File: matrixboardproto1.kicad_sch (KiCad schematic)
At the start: 11 parts, among them Q1 BC107, SW1 SW_Push

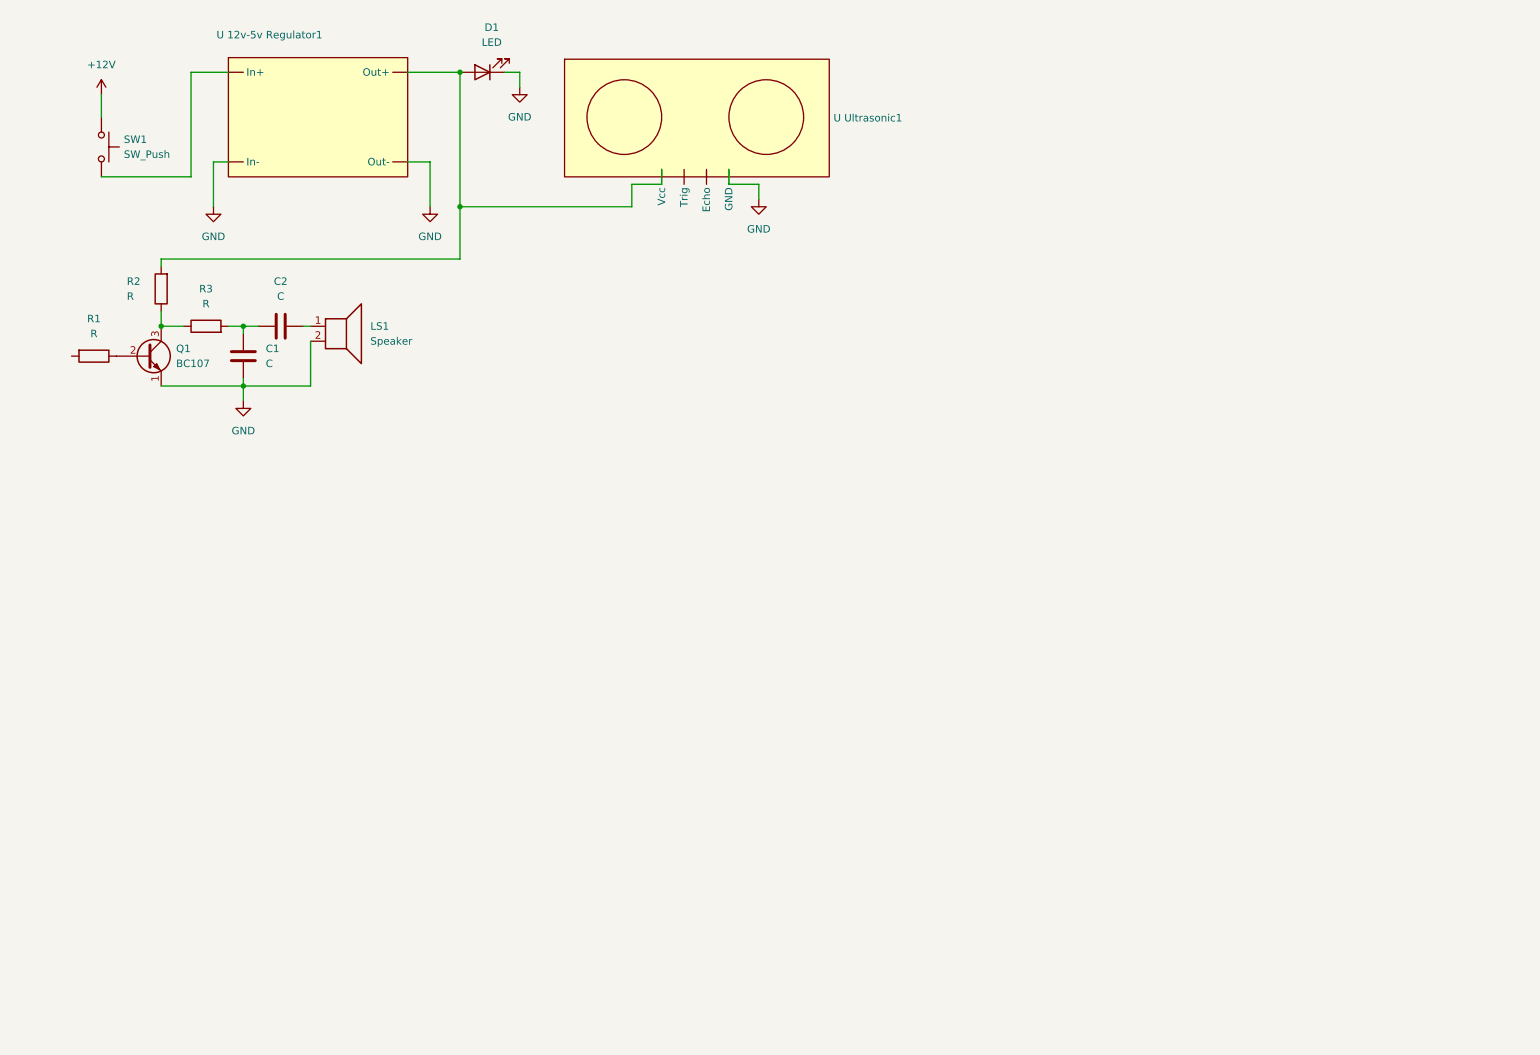
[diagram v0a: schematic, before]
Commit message: Add files via upload
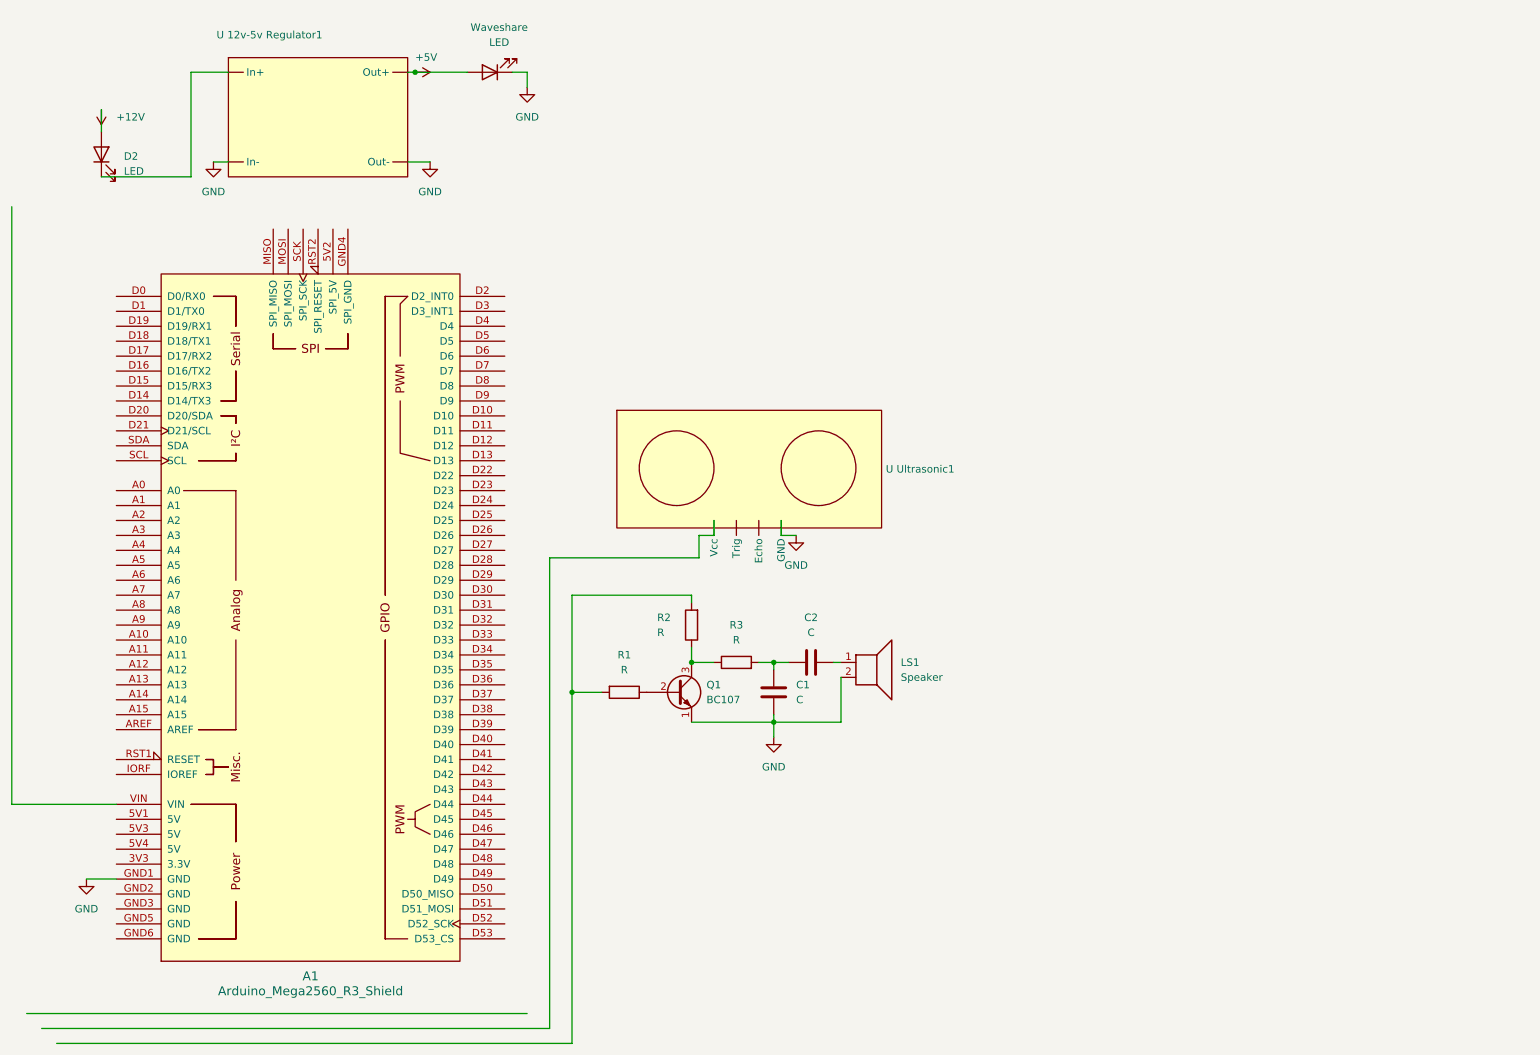
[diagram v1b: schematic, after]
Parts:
- removed SW1: SW_Push, symbol Switch:SW_Push
- added A1: Arduino_Mega2560_R3_Shield, PCM_arduino-library:Arduino_Mega2560_R3_Shield, symbol arduino-library:Arduino_Mega2560_R3_Shield
- added D2: LED, symbol Device:LED
- renumbered D1 to Waveshare
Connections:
- net +12V: now also D2.2 (A)
- net GND: now also A1.GND1 (GND)
- net at R1.2: now also R2.2
- new net: D2.1 (K), U 12v-5v Regulator1. (Out-)
- new net +5V: U 12v-5v Regulator1. (Out-), Waveshare.2 (A)
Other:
- moved on the sheet: C1, C2, LS1, Q1, R1, R2, R3, U Ultrasonic1, Waveshare

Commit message: Add files via upload
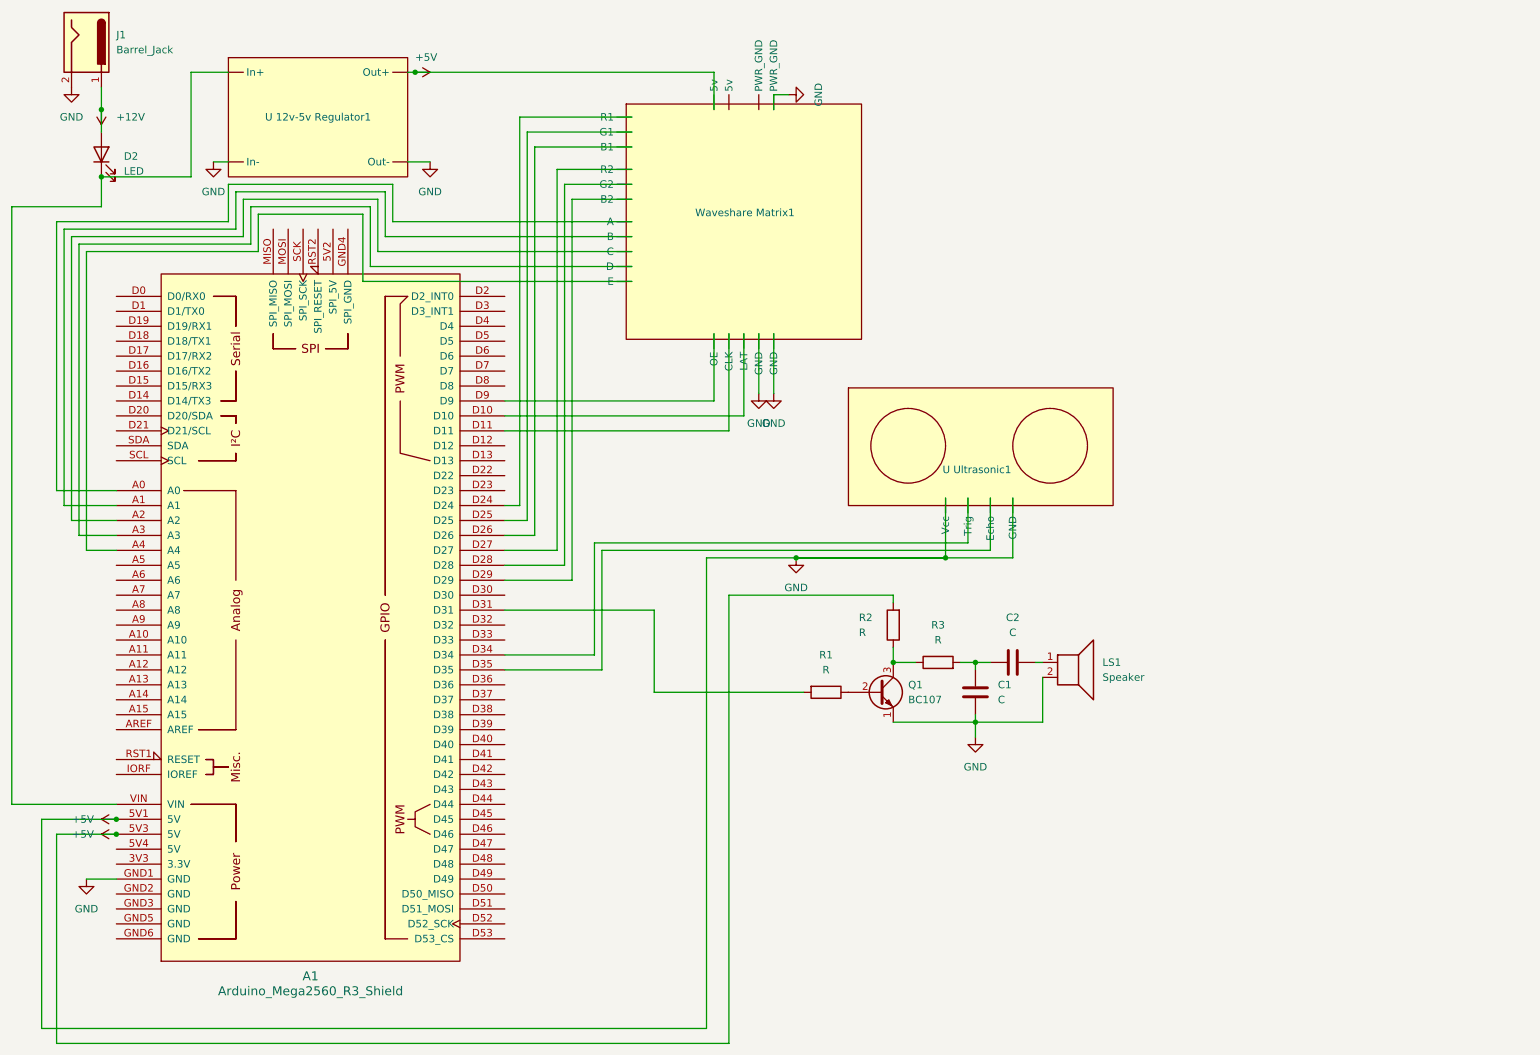
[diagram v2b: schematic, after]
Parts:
- removed Waveshare: LED, symbol Device:LED
- added J1: Barrel_Jack, symbol Connector:Barrel_Jack
- added Waveshare Matrix1: Waveshare Matrix, Waveshare Matrix, symbol Matrix_Board_Lib:Waveshare_LED_Matrix
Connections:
- net GND is gone; now on net +5V: A1.GND1 (GND), C1.1, LS1.2, Q1.1 (E), U 12v-5v Regulator1. (Out-), U Ultrasonic1. (Vcc)
- net +12V: now also J1.1
- net +5V: now also A1.5V1 (5V), A1.5V3 (5V), R2.2, J1.2, Waveshare Matrix1. (R2)
- net at D2.1 (K), U 12v-5v Regulator1. (Out-): now also A1.VIN
- net at R1.2: now also A1.D31; no longer R2.2
- net at A1.A0: now also Waveshare Matrix1. (R2)
- net at A1.A1: now also Waveshare Matrix1. (R2)
- net at A1.A2: now also Waveshare Matrix1. (R2)
- net at A1.A3: now also Waveshare Matrix1. (R2)
- net at A1.A4: now also Waveshare Matrix1. (R2)
- net at A1.D10: now also Waveshare Matrix1. (R2)
- net at A1.D11: now also Waveshare Matrix1. (R2)
- net at A1.D24: now also Waveshare Matrix1. (R2)
- net at A1.D25: now also Waveshare Matrix1. (R2)
- net at A1.D26: now also Waveshare Matrix1. (R2)
- net at A1.D27: now also Waveshare Matrix1. (R2)
- net at A1.D28: now also Waveshare Matrix1. (R2)
- net at A1.D29: now also Waveshare Matrix1. (R2)
- net at A1.D34: now also U Ultrasonic1. (Vcc)
- net at A1.D35: now also U Ultrasonic1. (Vcc)
- net at A1.D9: now also Waveshare Matrix1. (R2)
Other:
- moved on the sheet: C1, C2, LS1, Q1, R1, R2, R3, U Ultrasonic1

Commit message: Add files via upload
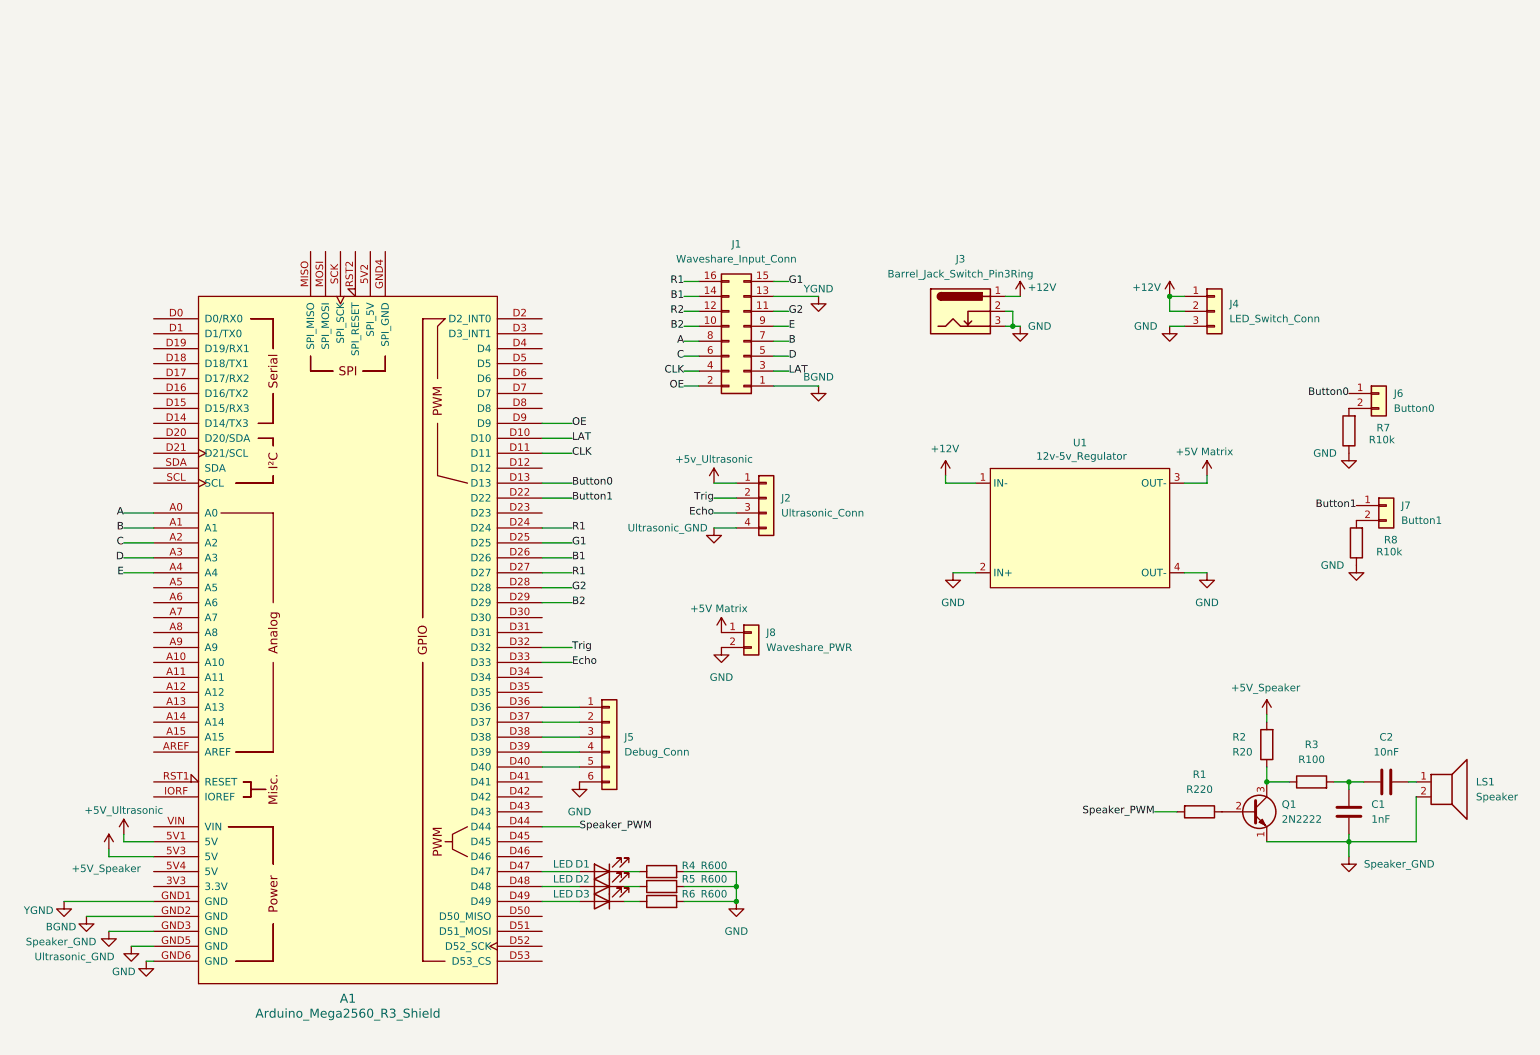
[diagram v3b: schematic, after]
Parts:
- removed J1: Barrel_Jack, symbol Connector:Barrel_Jack
- removed U 12v-5v Regulator1: ~, symbol Matrix_Board_Lib:DFR0831
- removed U Ultrasonic1: ~, symbol Matrix_Board_Lib:HCSR04_
- removed Waveshare Matrix1: Waveshare Matrix, Waveshare Matrix, symbol Matrix_Board_Lib:Waveshare_LED_Matrix
- added D1, D3: LED, LED_THT:LED_D5.0mm_Horizontal_O6.35mm_Z15.0mm, symbol Device:LED
- added J1: Waveshare_Input_Conn, Connector_IDC:IDC-Header_2x08_P2.54mm_Vertical, symbol Connector_Generic:Conn_02x08_Odd_Even
- added J2: Ultrasonic_Conn, Connector_PinHeader_1.00mm:PinHeader_1x04_P1.00mm_Vertical, symbol Connector_Generic:Conn_01x04
- added J3: Barrel_Jack_Switch_Pin3Ring, Connector_BarrelJack:BarrelJack_GCT_DCJ200-10-A_Horizontal, symbol Connector:Barrel_Jack_Switch_Pin3Ring
- added J4: LED_Switch_Conn, Connector:FanPinHeader_1x03_P2.54mm_Vertical, symbol Connector_Generic:Conn_01x03
- added J5: Debug_Conn, symbol Connector_Generic:Conn_01x06
- added J6: Button0, Connector_PinHeader_1.00mm:PinHeader_1x02_P1.00mm_Vertical, symbol Connector_Generic:Conn_01x02
- added J7: Button1, Connector_PinHeader_1.00mm:PinHeader_1x02_P1.00mm_Vertical, symbol Connector_Generic:Conn_01x02
- added J8: Waveshare_PWR, Connector_PinHeader_1.00mm:PinHeader_1x02_P1.00mm_Vertical, symbol Connector_Generic:Conn_01x02
- added R4, R5, R6: R600, Resistor_SMD:R_0805_2012Metric_Pad1.20x1.40mm_HandSolder, symbol Device:R
- added R7, R8: R10k, Resistor_SMD:R_0805_2012Metric_Pad1.20x1.40mm_HandSolder, symbol Device:R
- added U1: ~, matrixboard:DFR_Regulator, symbol Matrix_Board_Lib:DFR0831
- C1: value C -> 1nF; footprint (none) -> Capacitor_SMD:C_0805_2012Metric_Pad1.18x1.45mm_HandSolder
- C2: value C -> 10nF; footprint (none) -> Capacitor_SMD:C_0805_2012Metric_Pad1.18x1.45mm_HandSolder
- D2: footprint (none) -> LED_THT:LED_D5.0mm_Horizontal_O6.35mm_Z15.0mm
- LS1: footprint (none) -> Buzzer_Beeper:Speaker_CUI_CMR-1206S-67
- Q1: value BC107 -> 2N2222
- R1: value R -> R220; footprint (none) -> Resistor_SMD:R_0805_2012Metric_Pad1.20x1.40mm_HandSolder
- R2: value R -> R20; footprint (none) -> Resistor_SMD:R_0805_2012Metric_Pad1.20x1.40mm_HandSolder
- R3: value R -> R100; footprint (none) -> Resistor_SMD:R_0805_2012Metric_Pad1.20x1.40mm_HandSolder
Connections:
- net +12V: now also J3.1, J4.1 (Pin_1), J4.2 (Pin_2), U1.1 (IN-); no longer D2.2 (A)
- net at D2.1 (K): now also R5.1; no longer A1.VIN
- net A: now reaches A1.A0
- net A: now also J1.8 (Pin_8)
- net B: now reaches A1.A1
- net B: now also J1.7 (Pin_7)
- net C: now reaches A1.A2
- net C: now also J1.6 (Pin_6)
- net D: now reaches A1.A3
- net D: now also J1.5 (Pin_5)
- net E: now reaches A1.A4
- net E: now also J1.9 (Pin_9)
- net LAT: now reaches A1.D10
- net LAT: now also J1.3 (Pin_3)
- net CLK: now reaches A1.D11
- net CLK: now also J1.4 (Pin_4)
- net R1: now reaches A1.D24
- net R1: now also A1.D27, J1.16 (Pin_16)
- net G1: now reaches A1.D25
- net G1: now also J1.15 (Pin_15)
- net B1: now reaches A1.D26
- net B1: now also J1.14 (Pin_14)
- net G2: now reaches A1.D28
- net G2: now also J1.11 (Pin_11)
- net B2: now reaches A1.D29
- net B2: now also J1.10 (Pin_10)
- net OE: now reaches A1.D9
- net OE: now also J1.2 (Pin_2)
- net at A1.D31: no longer R1.2
- net Button0: now reaches A1.D13
- net Button0: now also J6.1 (Pin_1)
- net Button1: now reaches A1.D22
- net Button1: now also J7.1 (Pin_1)
- net Trig: now reaches A1.D32
- net Trig: now also J2.2 (Pin_2)
- net Echo: now reaches A1.D33
- net Echo: now also J2.3 (Pin_3)
- net at A1.D36: now also J5.1 (Pin_1)
- net at A1.D37: now also J5.2 (Pin_2)
- net at A1.D38: now also J5.3 (Pin_3)
- net at A1.D39: now also J5.4 (Pin_4)
- net at A1.D40: now also J5.5 (Pin_5)
- net Speaker_PWM: now reaches A1.D44
- net Speaker_PWM: now also R1.2
- net at A1.D47: now also D1.2 (A)
- net at A1.D48: now also D2.2 (A)
- net at A1.D49: now also D3.2 (A)
- net BGND: now reaches A1.GND2 (GND)
- net BGND: now also J1.1 (Pin_1)
- net Speaker_GND: now reaches A1.GND3 (GND)
- net Speaker_GND: now also C1.1, LS1.2, Q1.1 (E)
- net Ultrasonic_GND: now reaches A1.GND5 (GND)
- net Ultrasonic_GND: now also J2.4 (Pin_4)
- net GND: now reaches A1.GND6 (GND)
- net GND: now also J3.2, J3.3, J4.3 (Pin_3), J5.6 (Pin_6), J8.2 (Pin_2), R4.2, R5.2, R6.2, R7.1, R8.1, U1.2 (IN+), U1.4 (OUT-)
- removed net +5V: A1.5V1 (5V), A1.5V3 (5V), A1.GND1 (GND), C1.1, LS1.2, Q1.1 (E), R2.2
- new net: D3.1 (K), R6.1
- new net: J7.2 (Pin_2), R8.2
- new net: J6.2 (Pin_2), R7.2
- new net: D1.1 (K), R4.1
- new net +5V Matrix: J8.1 (Pin_1), U1.3 (OUT-)
- new net +5V_Speaker: A1.5V3 (5V), R2.2
- new net +5V_Ultrasonic: A1.5V1 (5V)
- new net +5v_Ultrasonic: J2.1 (Pin_1)
- new net R2: J1.12 (Pin_12)
- new net YGND: A1.GND1 (GND), J1.13 (Pin_13)
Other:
- note added: "12v-5v_Regulator"
- moved on the sheet: A1, C1, C2, LS1, Q1, R1, R2, R3
